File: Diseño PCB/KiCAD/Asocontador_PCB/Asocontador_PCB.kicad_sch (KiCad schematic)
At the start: 11 parts, among them J1 Screw_Terminal_2_P5.00mm, U1 LM7805_TO220

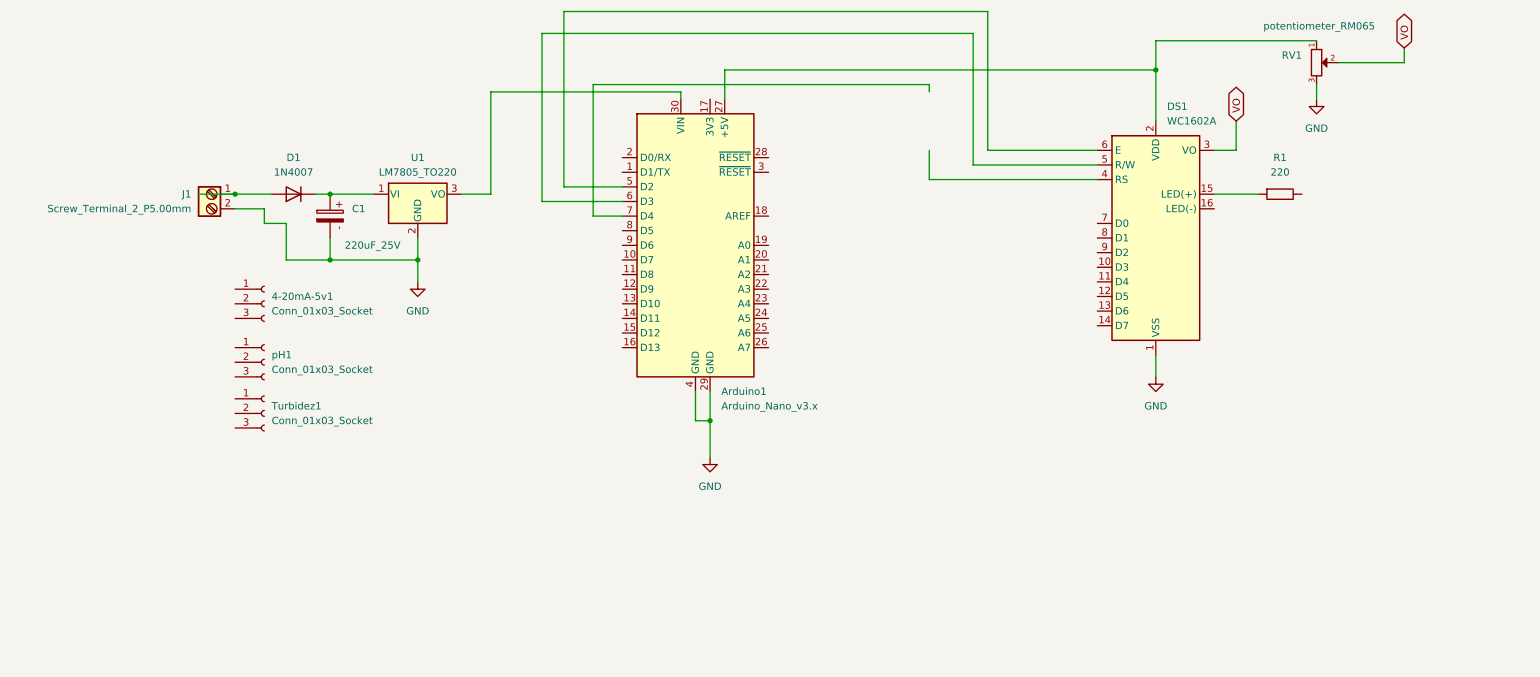
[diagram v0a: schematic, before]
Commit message: Modificaciones varias
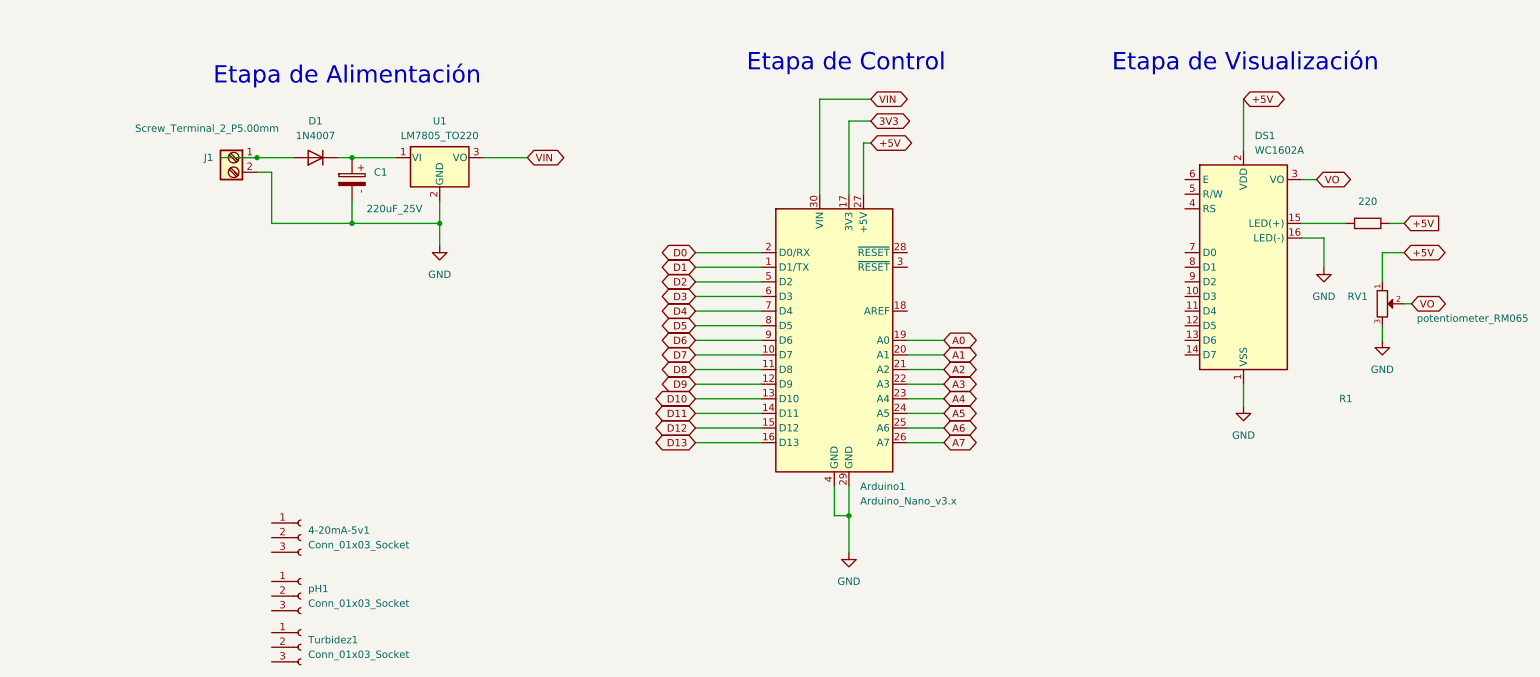
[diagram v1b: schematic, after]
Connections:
- net GND: now also DS1.16 (LED(-))
- net VIN: now reaches Arduino1.30 (VIN), U1.3 (VO)
- net +5V: now reaches Arduino1.27 (+5V), DS1.2 (VDD), RV1.1
- net +5V: now also R1.2
- net at DS1.5 (R/W): no longer Arduino1.6 (D3)
- net at DS1.6 (E): no longer Arduino1.5 (D2)
- net D1: now reaches Arduino1.1 (D1/TX)
- net D7: now reaches Arduino1.10 (D7)
- net D8: now reaches Arduino1.11 (D8)
- net D9: now reaches Arduino1.12 (D9)
- net D10: now reaches Arduino1.13 (D10)
- net D11: now reaches Arduino1.14 (D11)
- net D12: now reaches Arduino1.15 (D12)
- net D13: now reaches Arduino1.16 (D13)
- net 3V3: now reaches Arduino1.17 (3V3)
- net A0: now reaches Arduino1.19 (A0)
- net D0: now reaches Arduino1.2 (D0/RX)
- net A1: now reaches Arduino1.20 (A1)
- net A2: now reaches Arduino1.21 (A2)
- net A3: now reaches Arduino1.22 (A3)
- net A4: now reaches Arduino1.23 (A4)
- net A5: now reaches Arduino1.24 (A5)
- net A6: now reaches Arduino1.25 (A6)
- net A7: now reaches Arduino1.26 (A7)
- net D4: now reaches Arduino1.7 (D4)
- net D5: now reaches Arduino1.8 (D5)
- net D6: now reaches Arduino1.9 (D6)
- new net D2: Arduino1.5 (D2)
- new net D3: Arduino1.6 (D3)
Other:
- note added: "Etapa de Alimentación"
- note added: "Etapa de Control"
- note added: "Etapa de Visualización"
- moved on the sheet: 4-20mA-5v1, Arduino1, C1, D1, DS1, J1, R1, RV1, Turbidez1, U1, pH1
